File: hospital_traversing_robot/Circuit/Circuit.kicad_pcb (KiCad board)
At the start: 2 copper layers, 86.8 x 64 mm, 30 parts, among them J1 Barrel_Jack, U1 L7805, U2 L298N, U3 LD33v, U4 NRF24L01_Breakout

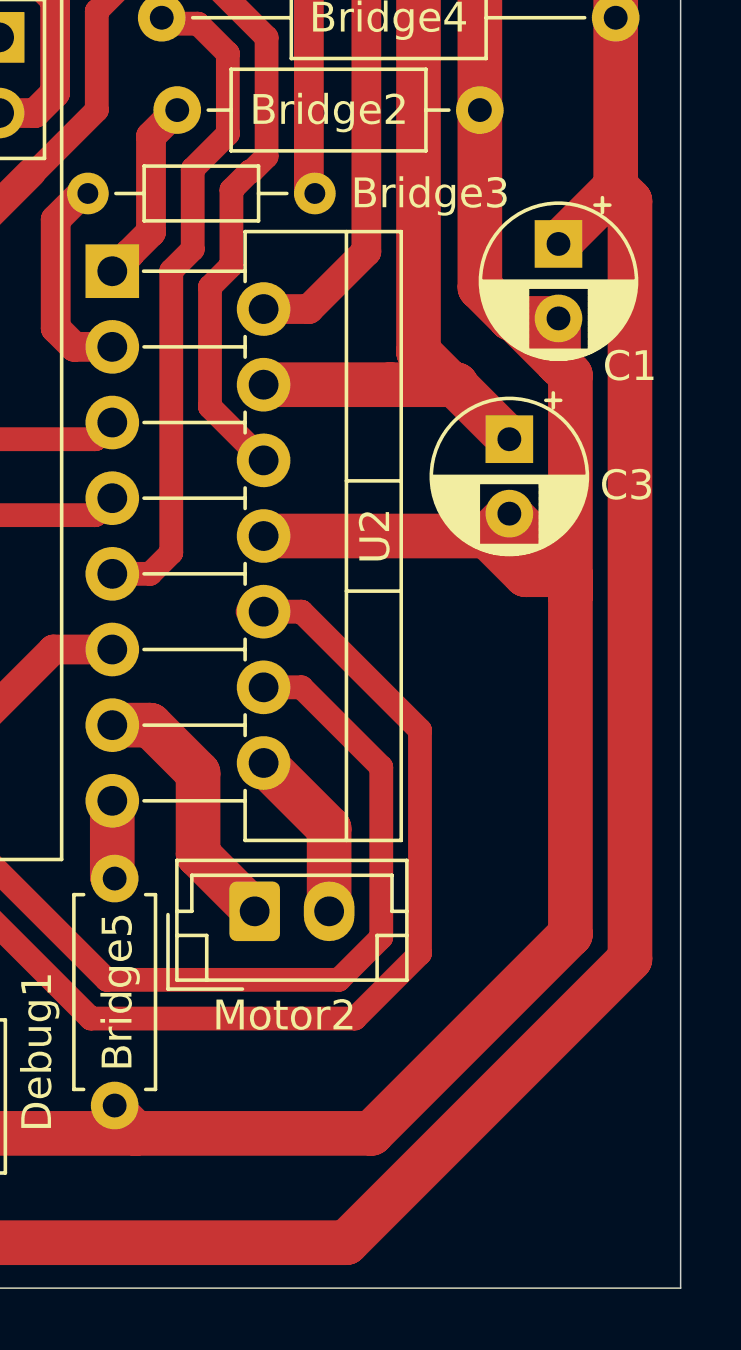
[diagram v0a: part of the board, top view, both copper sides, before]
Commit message: added circuit step files for both current projects
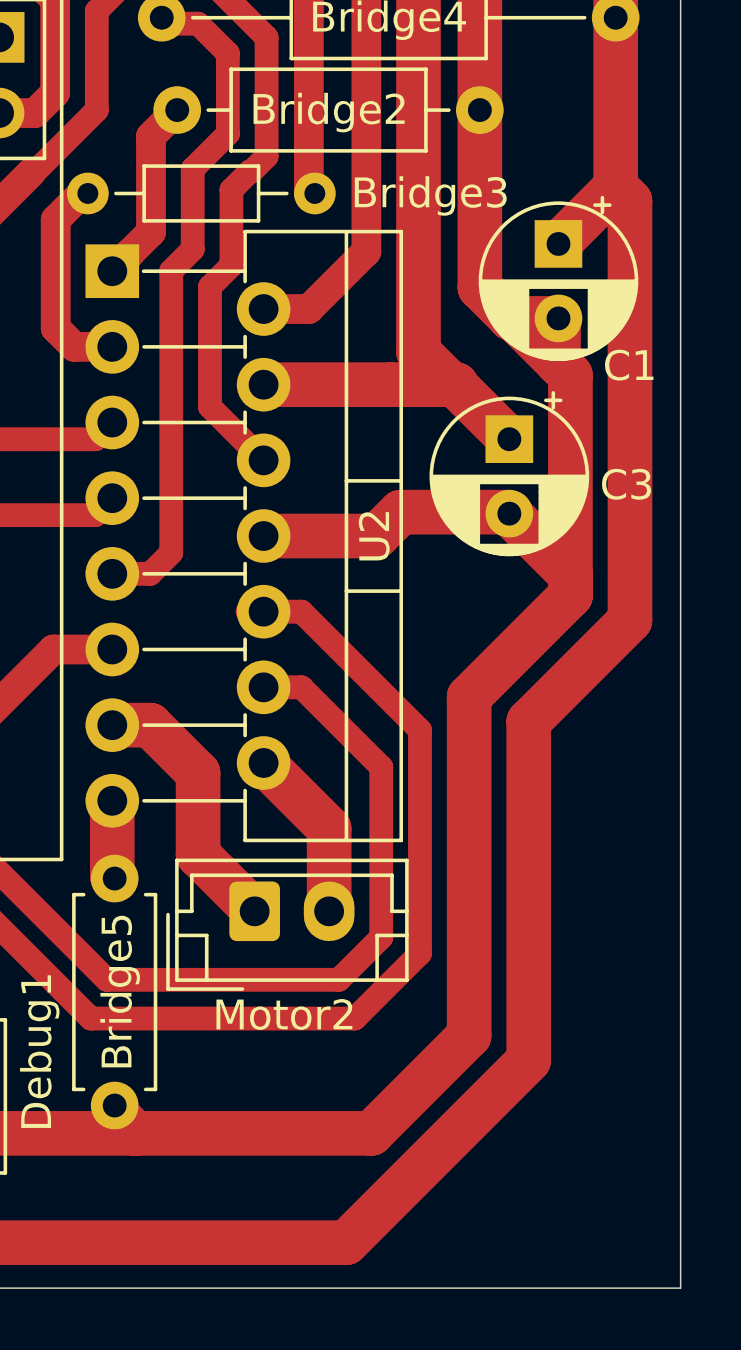
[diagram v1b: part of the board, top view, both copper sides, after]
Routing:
- net GND: track 301.4 -> 298.1 mm
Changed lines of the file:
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@@
-	)
-	(segment
-		(start 151.616572 105.055)
-		(end 158.3 98.371572)
-		(width 1.5)
-		(layer "F.Cu")
-		(net 2)
 	)
 	(segment
@@
 	)
 	(segment
+		(start 151.8 85)
+		(end 148 85)
+		(width 1.5)
+		(layer "F.Cu")
+		(net 2)
+	)
+	(segment
 		(start 109.25 54.506572)
 		(end 109.25 62.65)
@@
 	)
 	(segment
-		(start 158.3 98.371572)
-		(end 158.3 87)
-		(width 1.5)
-		(layer "F.Cu")
-		(net 2)
-	)
-	(segment
 		(start 116.3 99.54)
 		(end 116.7 99.54)
@@
 	)
 	(segment
+		(start 103.7 68.2)
+		(end 103.7 72.442081)
+		(width 1.5)
+		(layer "F.Cu")
+		(net 2)
+	)
+	(segment
+		(start 113.5 68.06)
+		(end 117.65 63.91)
+		(width 0.8)
+		(layer "F.Cu")
+		(net 2)
+	)
+	(segment
+		(start 156.3 77.694888)
+		(end 156.394888 77.694888)
+		(width 1.5)
+		(layer "F.Cu")
+		(net 2)
+	)
+	(segment
+		(start 103.7 72.442081)
+		(end 106.4 75.142081)
+		(width 1.5)
+		(layer "F.Cu")
+		(net 2)
+	)
+	(segment
+		(start 155.26 76.654888)
+		(end 156.3 77.694888)
+		(width 1.5)
+		(layer "F.Cu")
+		(net 2)
+	)
+	(segment
+		(start 155.26 60.588428)
+		(end 155.26 70.7)
+		(width 1.5)
+		(layer "F.Cu")
+		(net 2)
+	)
+	(segment
+		(start 152.6 84.2)
+		(end 151.8 85)
+		(width 1.5)
+		(layer "F.Cu")
+		(net 2)
+	)
+	(segment
+		(start 158.3 86.3)
+		(end 156.25 84.25)
+		(width 1.5)
+		(layer "F.Cu")
+		(net 2)
+	)
+	(segment
+		(start 158.3 87)
+		(end 158.3 86.3)
+		(width 1.5)
+		(layer "F.Cu")
+		(net 2)
+	)
+	(segment
+		(start 127.59 53.46)
+		(end 125.35 51.22)
+		(width 1.5)
+		(layer "F.Cu")
+		(net 2)
+	)
+	(segment
+		(start 114.58 71.14)
+		(end 113.5 70.06)
+		(width 0.8)
+		(layer "F.Cu")
+		(net 2)
+	)
+	(segment
+		(start 113.25 100.25)
+		(end 115.59 100.25)
+		(width 0.8)
+		(layer "F.Cu")
+		(net 2)
+	)
+	(segment
+		(start 156.394888 77.694888)
+		(end 157.9 79.2)
+		(width 1.5)
+		(layer "F.Cu")
+		(net 2)
+	)
+	(segment
+		(start 101.65104 106.528959)
+		(end 101.65104 99.95104)
+		(width 1.5)
+		(layer "F.Cu")
+		(net 2)
+	)
+	(segment
 		(start 143.7 105.055)
 		(end 151.616572 105.055)
@@
 	)
 	(segment
-		(start 103.7 68.2)
-		(end 103.7 72.442081)
-		(width 1.5)
-		(layer "F.Cu")
-		(net 2)
-	)
-	(segment
-		(start 156.8 86.3)
-		(end 158.3 86.3)
-		(width 1.5)
-		(layer "F.Cu")
-		(net 2)
-	)
-	(segment
-		(start 113.5 68.06)
-		(end 117.65 63.91)
-		(width 0.8)
-		(layer "F.Cu")
-		(net 2)
-	)
-	(segment
-		(start 156.3 77.694888)
-		(end 156.394888 77.694888)
-		(width 1.5)
-		(layer "F.Cu")
-		(net 2)
-	)
-	(segment
-		(start 103.7 72.442081)
-		(end 106.4 75.142081)
-		(width 1.5)
-		(layer "F.Cu")
-		(net 2)
-	)
-	(segment
-		(start 155.26 76.654888)
-		(end 156.3 77.694888)
-		(width 1.5)
-		(layer "F.Cu")
-		(net 2)
-	)
-	(segment
-		(start 155.26 60.588428)
-		(end 155.26 70.7)
-		(width 1.5)
-		(layer "F.Cu")
-		(net 2)
-	)
-	(segment
-		(start 158.3 87)
-		(end 158.3 86.3)
-		(width 1.5)
-		(layer "F.Cu")
-		(net 2)
-	)
-	(segment
-		(start 127.59 53.46)
-		(end 125.35 51.22)
-		(width 1.5)
-		(layer "F.Cu")
-		(net 2)
-	)
-	(segment
-		(start 114.58 71.14)
-		(end 113.5 70.06)
-		(width 0.8)
-		(layer "F.Cu")
-		(net 2)
-	)
-	(segment
-		(start 158.3 86.3)
-		(end 156.25 84.25)
-		(width 1.5)
-		(layer "F.Cu")
-		(net 2)
-	)
-	(segment
-		(start 113.25 100.25)
-		(end 115.59 100.25)
-		(width 0.8)
-		(layer "F.Cu")
-		(net 2)
-	)
-	(segment
-		(start 156.394888 77.694888)
-		(end 157.9 79.2)
-		(width 1.5)
-		(layer "F.Cu")
-		(net 2)
-	)
-	(segment
-		(start 101.65104 106.528959)
-		(end 101.65104 99.95104)
-		(width 1.5)
-		(layer "F.Cu")
-		(net 2)
-	)
-	(segment
 		(start 143 104.355)
 		(end 143.7 105.055)
@@
 	)
 	(segment
-		(start 155.5 85)
-		(end 156.8 86.3)
-		(width 1.5)
-		(layer "F.Cu")
-		(net 2)
-	)
-	(segment
 		(start 126.35 54.7)
 		(end 127.59 53.46)
@@
 	)
 	(segment
-		(start 155.5 85)
-		(end 148 85)
-		(width 1.5)
-		(layer "F.Cu")
-		(net 2)
-	)
-	(segment
 		(start 134.77 63.91)
 		(end 139.12 68.26)
@@
 	)
 	(segment
+		(start 154.9 90.4)
+		(end 158.3 87)
+		(width 1.5)
+		(layer "F.Cu")
+		(net 2)
+	)
+	(segment
+		(start 156.2 84.2)
+		(end 152.6 84.2)
+		(width 1.5)
+		(layer "F.Cu")
+		(net 2)
+	)
+	(segment
 		(start 112.536572 51.22)
 		(end 109.25 54.506572)
@@
 	)
 	(segment
+		(start 154.9 101.771572)
+		(end 154.9 90.4)
+		(width 1.5)
+		(layer "F.Cu")
+		(net 2)
+	)
+	(segment
 		(start 158.3 79.6)
 		(end 157.9 79.2)
@@
 	)
 	(segment
+		(start 151.616572 105.055)
+		(end 154.9 101.771572)
+		(width 1.5)
+		(layer "F.Cu")
+		(net 2)
+	)
+	(segment
 		(start 101.65104 79.891041)
 		(end 101.65104 97.65104)
@@
 	)
 	(segment
+		(start 156.25 84.25)
+		(end 156.2 84.2)
+		(width 1.5)
+		(layer "F.Cu")
+		(net 2)
+	)
+	(segment
 		(start 103.65104 108.528959)
 		(end 101.65104 106.528959)
@@
 		(start 138.8 53.46)
 		(end 148.131572 53.46)
-		(width 1.5)
-		(layer "F.Cu")
-		(net 2)
-	)
-	(segment
-		(start 156.25 84.25)
-		(end 155.5 85)
 		(width 1.5)
 		(layer "F.Cu")
@@
 	)
 	(segment
-		(start 150.775 108.725)
-		(end 127.130152 108.725)
-		(width 1.5)
-		(layer "F.Cu")
-		(net 4)
-	)
-	(segment
-		(start 160.3 73.754888)
-		(end 160.3 99.2)
+		(start 159.82 73.274888)
+		(end 160.3 73.754888)
 		(width 1.5)
 		(layer "F.Cu")
@@
 		(start 138.8 50.92)
 		(end 148.42 50.92)
+		(width 1.5)
+		(layer "F.Cu")
+		(net 4)
+	)
+	(segment
+		(start 160.3 87.828428)
+		(end 156.9 91.228428)
+		(width 1.5)
+		(layer "F.Cu")
+		(net 4)
+	)
+	(segment
+		(start 127.130152 108.725)
+		(end 125.5 107.094848)
 		(width 1.5)
 		(layer "F.Cu")
@@
 	)
 	(segment
+		(start 125.5 107.094848)
+		(end 125.5 106.5)
+		(width 1.5)
+		(layer "F.Cu")
+		(net 4)
+	)
+	(segment
+		(start 160.3 73.754888)
+		(end 160.3 87.828428)
+		(width 1.5)
+		(layer "F.Cu")
+		(net 4)
+	)
+	(segment
 		(start 159.82 67.6)
 		(end 159.82 73.274888)
@@
 	)
 	(segment
-		(start 159.82 73.274888)
-		(end 160.3 73.754888)
-		(width 1.5)
-		(layer "F.Cu")
-		(net 4)
-	)
-	(segment
 		(start 159.82 62.32)
 		(end 159.82 67.6)
@@
 	)
 	(segment
-		(start 127.130152 108.725)
-		(end 125.5 107.094848)
-		(width 1.5)
-		(layer "F.Cu")
-		(net 4)
-	)
-	(segment
 		(start 148.42 50.92)
 		(end 159.82 62.32)
@@
 	)
 	(segment
+		(start 150.775 108.725)
+		(end 127.130152 108.725)
+		(width 1.5)
+		(layer "F.Cu")
+		(net 4)
+	)
+	(segment
+		(start 156.9 102.6)
+		(end 150.775 108.725)
+		(width 1.5)
+		(layer "F.Cu")
+		(net 4)
+	)
+	(segment
 		(start 159.82 73.274888)
 		(end 157.9 75.194888)
@@
 	)
 	(segment
-		(start 125.5 107.094848)
-		(end 125.5 106.5)
-		(width 1.5)
-		(layer "F.Cu")
-		(net 4)
-	)
-	(segment
-		(start 160.3 99.2)
-		(end 150.775 108.725)
-		(width 1.5)
-		(layer "F.Cu")
+		(start 156.9 91.228428)
+		(end 156.9 102.6)
+		(width 1.5)
+		(layer "F.Cu")
